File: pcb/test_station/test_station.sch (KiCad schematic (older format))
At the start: 10 parts

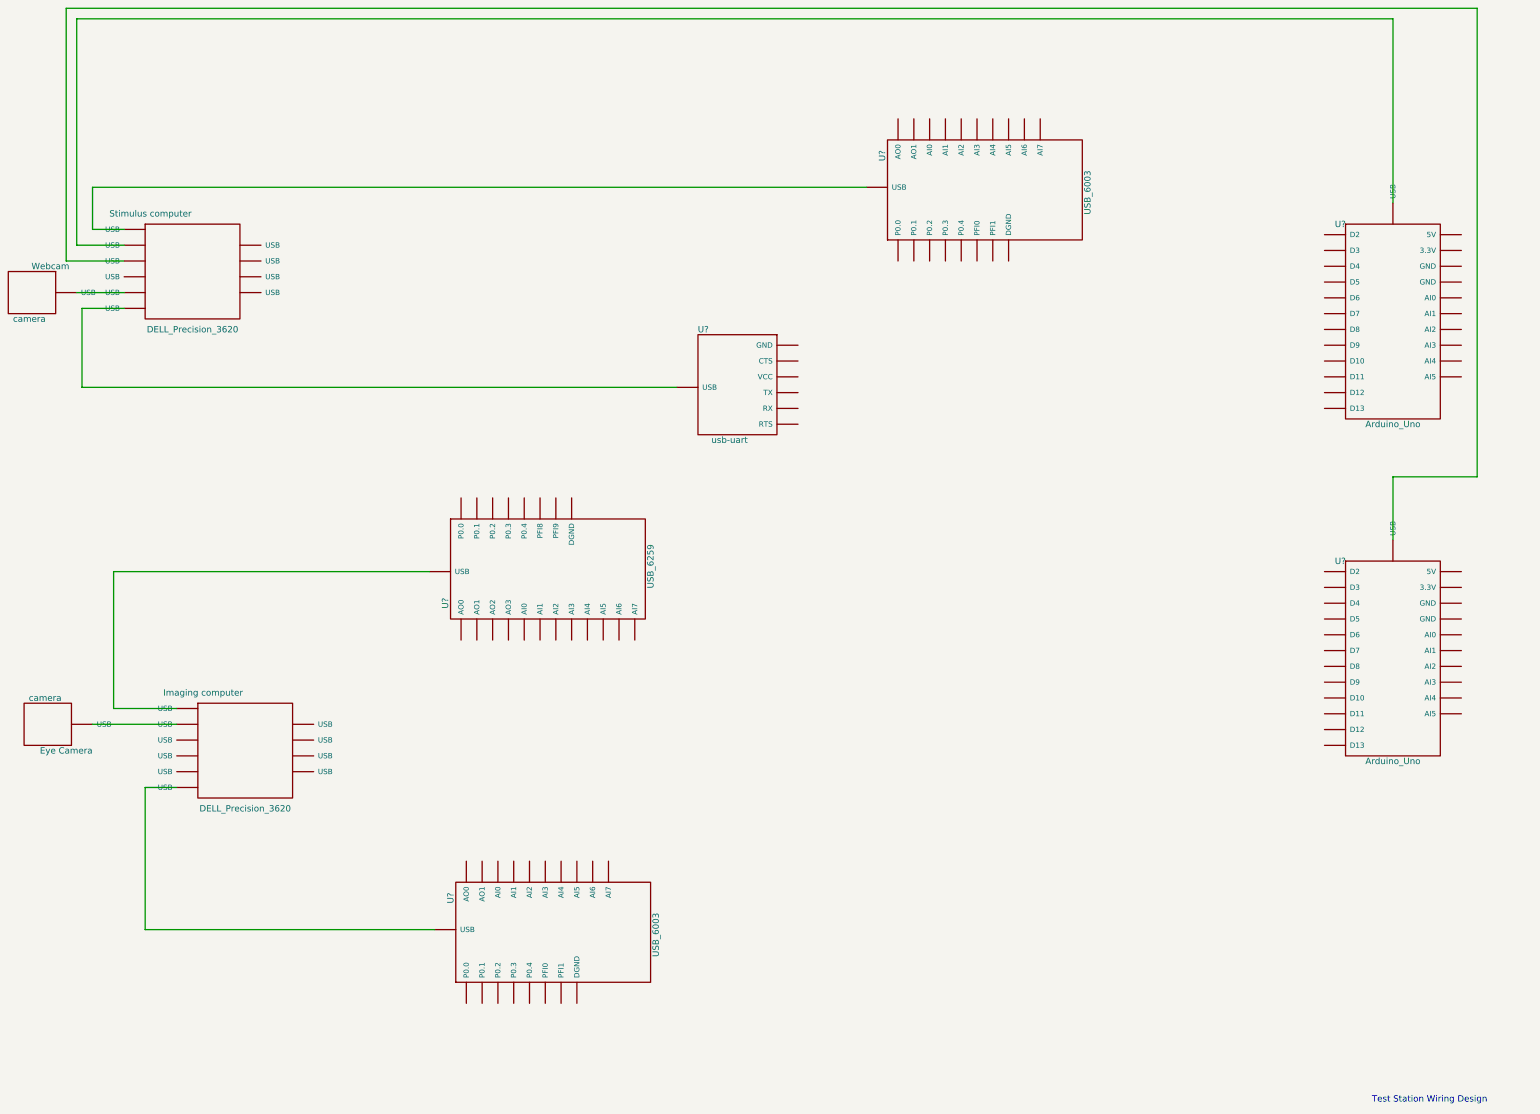
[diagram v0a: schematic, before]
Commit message: some progress with test station wiring
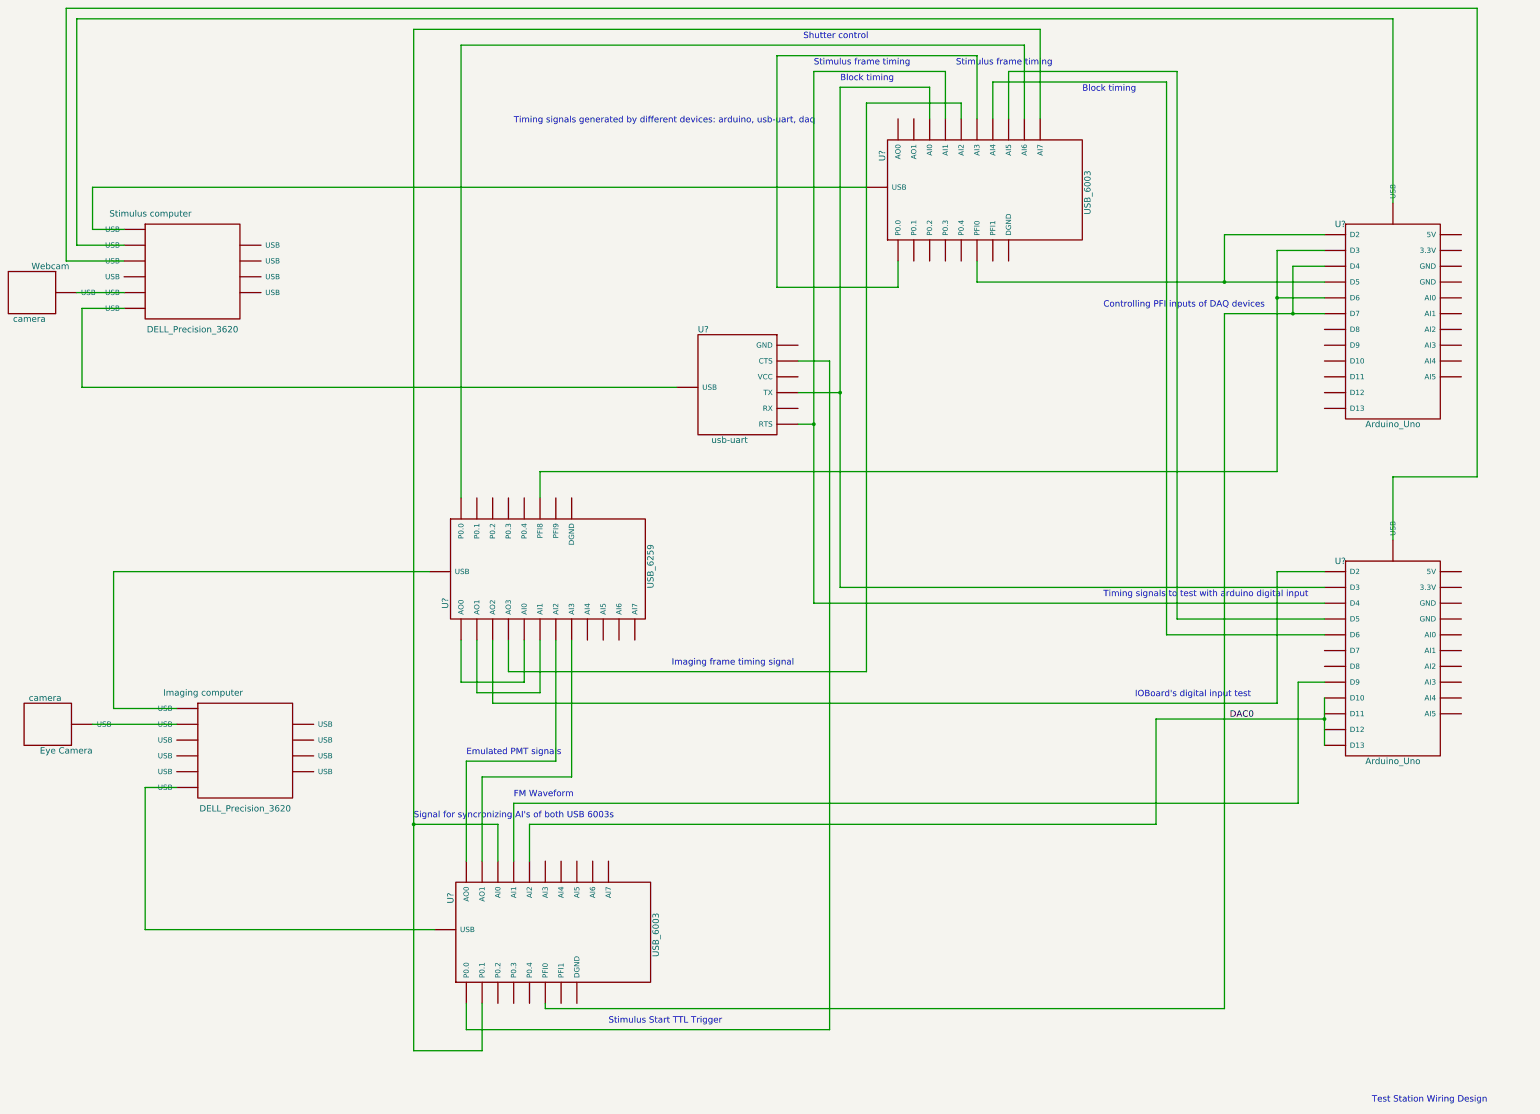
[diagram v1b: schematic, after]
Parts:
- renumbered Eye to Eye~Camera, Imaging to Imaging~computer, Stimulus to Stimulus~computer
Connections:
- net labels added: DAC0
- wire segments 24 -> 106
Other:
- note added: "Block timing"
- note added: "Controlling PFI inputs of DAQ devices"
- note added: "Emulated PMT signals"
- note added: "FM Waveform"
- note added: "IOBoard's digital input test"
- note added: "Imaging frame timing signal"
- note added: "Shutter control"
- note added: "Signal for syncronizing AI's of both USB 6003s"
- note added: "Stimulus Start TTL Trigger"
- note added: "Stimulus frame timing"
- note added: "Timing signals generated by different devices: arduino, usb-uart, daq"
- note added: "Timing signals to test with arduino digital input"
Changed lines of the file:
@@
 LIBS:valves
 LIBS:test_station_components
+LIBS:test_station-cache
 EELAYER 25 0
 EELAYER END
@@
 $EndDescr
 $Comp
-L DELL_Precision_3620 Stimulus
+L DELL_Precision_3620 Stimulus~computer
 U 1 1 5A73450C
 P 2450 3200
@@
 $EndComp
 $Comp
-L DELL_Precision_3620 Imaging
+L DELL_Precision_3620 Imaging~computer
 U 1 1 5A7345F9
 P 2950 7750
@@
 $EndComp
 $Comp
-L camera Eye
+L camera Eye~Camera
 U 1 1 5A7347A2
 P 1100 7300
@@
 	1    0    0    -1
 $EndComp
-Wire Wire Line
-	4700 5850 1700 5850
-Wire Wire Line
-	1700 5850 1700 7150
-Wire Wire Line
-	1700 7150 2300 7150
-Wire Wire Line
-	1500 7300 2300 7300
-Wire Wire Line
-	4750 9250 2000 9250
-Wire Wire Line
-	2000 9250 2000 7900
-Wire Wire Line
-	2000 7900 2300 7900
-Wire Wire Line
-	7050 4100 1400 4100
-Wire Wire Line
-	1400 4100 1400 3350
-Wire Wire Line
-	1400 3350 1800 3350
-Wire Wire Line
-	1800 3200 1350 3200
-Wire Wire Line
-	8850 2200 1500 2200
-Wire Wire Line
-	1500 2200 1500 2600
-Wire Wire Line
-	1500 2600 1800 2600
-Wire Wire Line
-	1800 2750 1350 2750
-Wire Wire Line
-	1350 2750 1350 600
-Wire Wire Line
-	1350 600  13850 600
-Wire Wire Line
-	13850 600  13850 2350
-Wire Wire Line
-	13850 5550 13850 4950
-Wire Wire Line
-	13850 4950 14650 4950
-Wire Wire Line
-	14650 4950 14650 500
-Wire Wire Line
-	14650 500  1250 500
-Wire Wire Line
-	1250 500  1250 2900
-Wire Wire Line
-	1250 2900 1800 2900
 Text Notes 13650 10900 0    60   ~ 0
 Test Station Wiring Design
+Text Label 12300 7250 0    60   ~ 0
+DAC0
+Text Notes 6400 10150 0    60   ~ 0
+Stimulus Start TTL Trigger
+Text Notes 11400 7050 0    60   ~ 0
+IOBoard's digital input test
+Text Notes 7000 6750 0    60   ~ 0
+Imaging frame timing signal
+Text Notes 8350 1050 0    60   ~ 0
+Stimulus frame timing
+Text Notes 8600 1200 0    60   ~ 0
+Block timing
+Text Notes 9700 1050 0    60   ~ 0
+Stimulus frame timing
+Text Notes 10900 1300 0    60   ~ 0
+Block timing
+Text Notes 11100 6100 0    60   ~ 0
+Timing signals to test with arduino digital input
+Text Notes 8250 800  0    60   ~ 0
+Shutter control
+Text Notes 5500 8000 0    60   ~ 0
+FM Waveform
+Wire Wire Line
+	4700 5850 1700 5850
+Wire Wire Line
+	1700 5850 1700 7150
+Wire Wire Line
+	1700 7150 2300 7150
+Wire Wire Line
+	1500 7300 2300 7300
+Wire Wire Line
+	4750 9250 2000 9250
+Wire Wire Line
+	2000 9250 2000 7900
+Wire Wire Line
+	2000 7900 2300 7900
+Wire Wire Line
+	7050 4100 1400 4100
+Wire Wire Line
+	1400 4100 1400 3350
+Wire Wire Line
+	1400 3350 1800 3350
+Wire Wire Line
+	1800 3200 1350 3200
+Wire Wire Line
+	8850 2200 1500 2200
+Wire Wire Line
+	1500 2200 1500 2600
+Wire Wire Line
+	1500 2600 1800 2600
+Wire Wire Line
+	1800 2750 1350 2750
+Wire Wire Line
+	1350 2750 1350 600
+Wire Wire Line
+	1350 600  13850 600
+Wire Wire Line
+	13850 600  13850 2350
+Wire Wire Line
+	13850 5550 13850 4950
+Wire Wire Line
+	13850 4950 14650 4950
+Wire Wire Line
+	14650 4950 14650 500
+Wire Wire Line
+	14650 500  1250 500
+Wire Wire Line
+	1250 500  1250 2900
+Wire Wire Line
+	1250 2900 1800 2900
+Wire Wire Line
+	5000 6500 5000 6900
+Wire Wire Line
+	5000 6900 5600 6900
+Wire Wire Line
+	5600 6900 5600 6500
+Wire Wire Line
+	5150 6500 5150 7000
+Wire Wire Line
+	5150 7000 5750 7000
+Wire Wire Line
+	5750 7000 5750 6500
+Wire Wire Line
+	13200 7050 13200 7500
+Wire Wire Line
+	13200 7250 11600 7250
+Connection ~ 13200 7250
+Wire Wire Line
+	5050 9950 5050 10200
+Wire Wire Line
+	5050 10200 8500 10200
+Wire Wire Line
+	8500 10200 8500 3850
+Wire Wire Line
+	8500 3850 8200 3850
+Wire Wire Line
+	5300 6500 5300 7100
+Wire Wire Line
+	5300 7100 12750 7100
+Wire Wire Line
+	12750 7100 12750 5850
+Wire Wire Line
+	12750 5850 13200 5850
+Wire Wire Line
+	5450 6500 5450 6800
+Wire Wire Line
+	5450 6800 8850 6800
+Wire Wire Line
+	8850 1400 9750 1400
+Wire Wire Line
+	8850 6800 8850 1400
+Wire Wire Line
+	8200 4150 8600 4150
+Wire Wire Line
+	8600 1250 8600 6000
+Wire Wire Line
+	8600 1250 9450 1250
+Wire Wire Line
+	8200 4450 8350 4450
+Wire Wire Line
+	8350 1100 8350 6150
+Wire Wire Line
+	8350 1100 9600 1100
+Wire Wire Line
+	13200 6300 11800 6300
+Wire Wire Line
+	11800 6300 11800 1100
+Wire Wire Line
+	11800 1100 10200 1100
+Wire Wire Line
+	13200 6450 11700 6450
+Wire Wire Line
+	11700 6450 11700 1200
+Wire Wire Line
+	11700 1200 10050 1200
+Wire Wire Line
+	9750 1400 9750 1550
+Wire Wire Line
+	9600 1100 9600 1550
+Wire Wire Line
+	9450 1250 9450 1550
+Wire Wire Line
+	8350 6150 13200 6150
+Connection ~ 8350 4450
+Wire Wire Line
+	8600 6000 13200 6000
+Connection ~ 8600 4150
+Wire Wire Line
+	9900 950  9900 1550
+Wire Wire Line
+	10050 1200 10050 1550
+Wire Wire Line
+	10200 1100 10200 1550
+Wire Wire Line
+	5000 5150 5000 850
+Wire Wire Line
+	5000 850  10350 850
+Wire Wire Line
+	10350 850  10350 1550
+Wire Wire Line
+	13200 6900 12950 6900
+Wire Wire Line
+	12950 6900 12950 8050
+Wire Wire Line
+	12950 8050 5500 8050
+Wire Wire Line
+	6050 6500 6050 7800
+Wire Wire Line
+	6050 7800 5200 7800
+Wire Wire Line
+	5200 7800 5200 8600
+Wire Wire Line
+	5900 6500 5900 7650
+Wire Wire Line
+	5900 7650 5050 7650
+Wire Wire Line
+	5050 7650 5050 8600
+Text Notes 5050 7600 0    60   ~ 0
+Emulated PMT signals
+Wire Wire Line
+	5200 9950 5200 10400
+Wire Wire Line
+	4550 10400 5200 10400
+Wire Wire Line
+	4550 700  4550 10400
+Wire Wire Line
+	4550 8250 5350 8250
+Wire Wire Line
+	5350 8250 5350 8600
+Text Notes 4550 8200 0    60   ~ 0
+Signal for syncronizing AI's of both USB 6003s
+Wire Wire Line
+	10500 1550 10500 700
+Wire Wire Line
+	10500 700  4550 700
+Connection ~ 4550 8250
+Wire Wire Line
+	5500 8050 5500 8600
+Wire Wire Line
+	9900 2900 9900 3100
+Wire Wire Line
+	5750 5150 5750 4900
+Wire Wire Line
+	12750 4900 5750 4900
+Wire Wire Line
+	12750 2800 12750 4900
+Wire Wire Line
+	12750 3250 13200 3250
+Wire Wire Line
+	9900 3100 13200 3100
+Wire Wire Line
+	5800 9950 5800 10000
+Wire Wire Line
+	5800 10000 12250 10000
+Wire Wire Line
+	12250 10000 12250 3400
+Wire Wire Line
+	12250 3400 13200 3400
+Wire Wire Line
+	13200 2650 12250 2650
+Wire Wire Line
+	12250 2650 12250 3100
+Connection ~ 12250 3100
+Wire Wire Line
+	12750 2800 13200 2800
+Connection ~ 12750 3250
+Wire Wire Line
+	13200 2950 12900 2950
+Wire Wire Line
+	12900 2950 12900 3400
+Connection ~ 12900 3400
+Text Notes 11100 3350 0    60   ~ 0
+Controlling PFI inputs of DAQ devices
+Wire Wire Line
+	5650 8600 5650 8250
+Wire Wire Line
+	5650 8250 11600 8250
+Wire Wire Line
+	11600 8250 11600 7250
+Wire Wire Line
+	9150 2900 9150 3150
+Wire Wire Line
+	9150 3150 8000 3150
+Wire Wire Line
+	8000 3150 8000 950
+Wire Wire Line
+	8000 950  9900 950
+Text Notes 5500 1600 0    60   ~ 0
+Timing signals generated by different devices: arduino, usb-uart, daq
 $EndSCHEMATC
